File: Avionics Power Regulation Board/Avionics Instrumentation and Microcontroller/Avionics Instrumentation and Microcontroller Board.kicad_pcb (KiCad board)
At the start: 2 copper layers, 101.9 x 63.6 mm, 18 parts, among them J1 Conn_01x04_Socket, J2 Conn_01x07_Socket, J3 Conn_01x06_Socket, J4 Conn_01x08_Socket, J5 Conn_01x05_Socket, J6 Conn_02x07_Odd_Even, J7 Micro_SD_Card_Det1, U1 SC0917

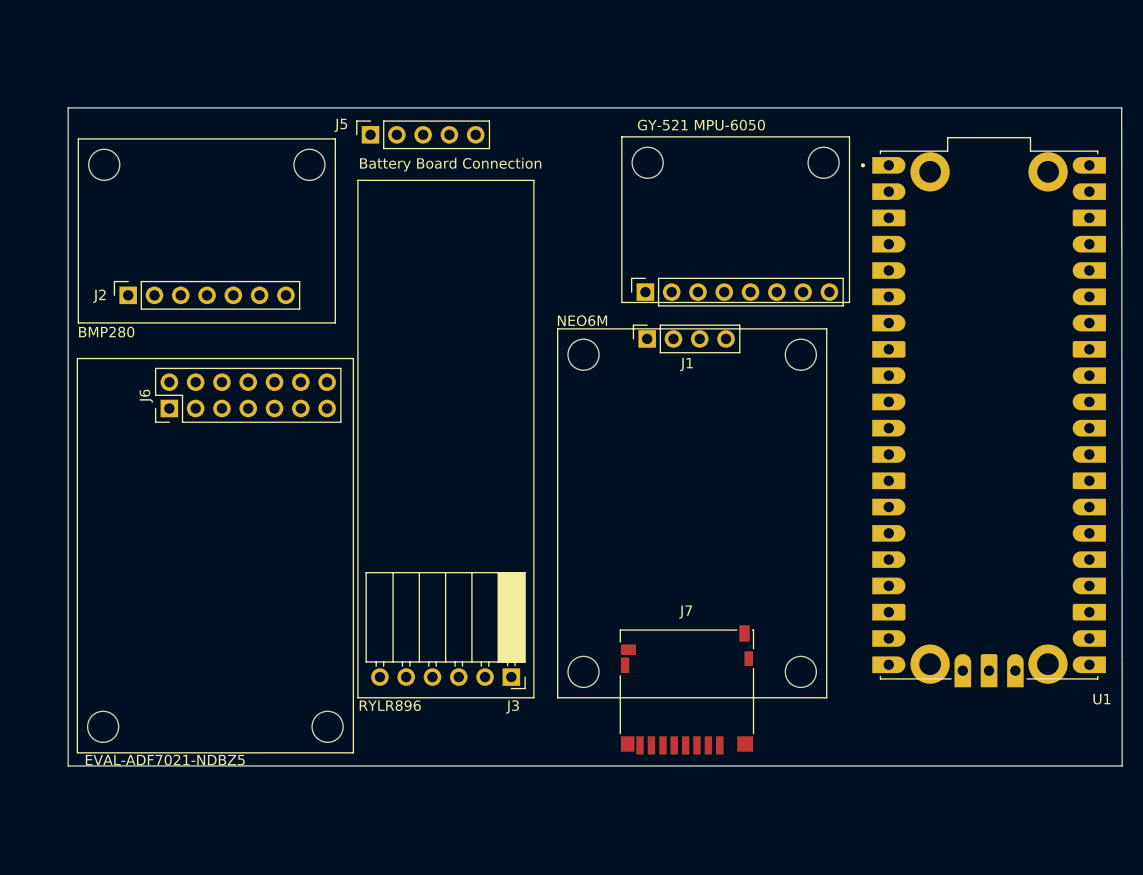
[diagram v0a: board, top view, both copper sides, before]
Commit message: Small Changes
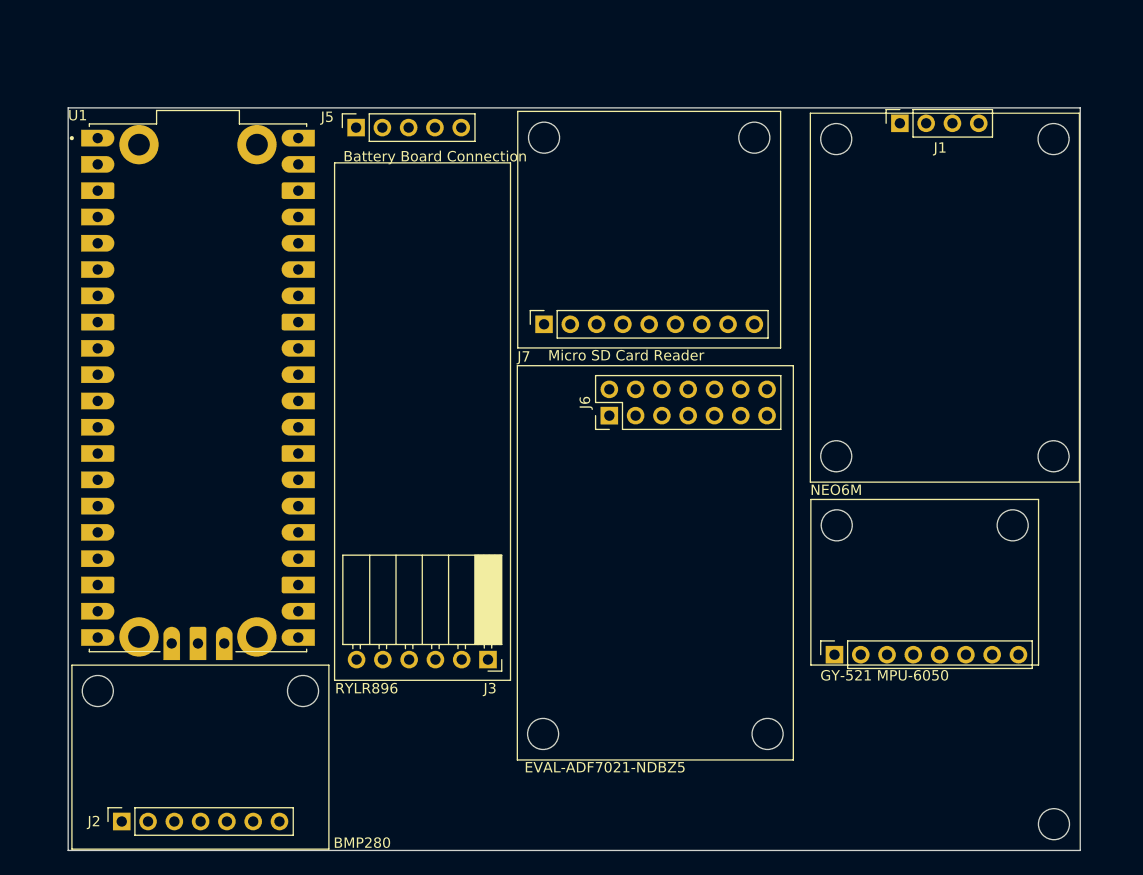
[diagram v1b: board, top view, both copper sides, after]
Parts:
- added H12: MountingHole, MountingHole:MountingHole_2.1mm, F.Cu at (80.3, 29.0)
- added H13: MountingHole, MountingHole:MountingHole_2.1mm, F.Cu at (100.6, 29.0)
- added H2: MountingHole, MountingHole:MountingHole_2.1mm, F.Cu at (129.5, 95.4)
- J7: value Micro_SD_Card_Det1 -> Conn_01x09_Socket; footprint Connector_Card:microSD_HC_Hirose_DM3D-SF -> Connector_PinSocket_2.54mm:PinSocket_1x09_P2.54mm_Vertical
- moved U1 76.5 mm to (46.8, 53.2)
- moved H1 50.8 mm to (37.1, 82.5)
- moved H7 50.8 mm to (57.0, 82.5)
- moved J2 50.8 mm to (39.5, 95.1)
- moved H11 42.5 mm to (80.2, 86.7)
- moved J6 42.5 mm to (86.6, 55.9)
- moved H8 42.5 mm to (101.9, 86.7)
- moved H10 39.5 mm to (125.5, 66.5)
- moved H9 39.5 mm to (108.5, 66.5)
- moved J4 39.5 mm to (108.3, 79.0)
- moved J7 37.9 mm to (80.3, 47.1), turned to 90 degrees
- moved H3 32.1 mm to (108.5, 29.2)
- moved H5 32.1 mm to (129.5, 29.2)
- moved H4 32.1 mm to (108.5, 59.8)
- moved H6 32.1 mm to (129.5, 59.8)
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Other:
- board size 101.9 x 63.6 mm -> 97.8 x 71.8 mm

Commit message: more changes
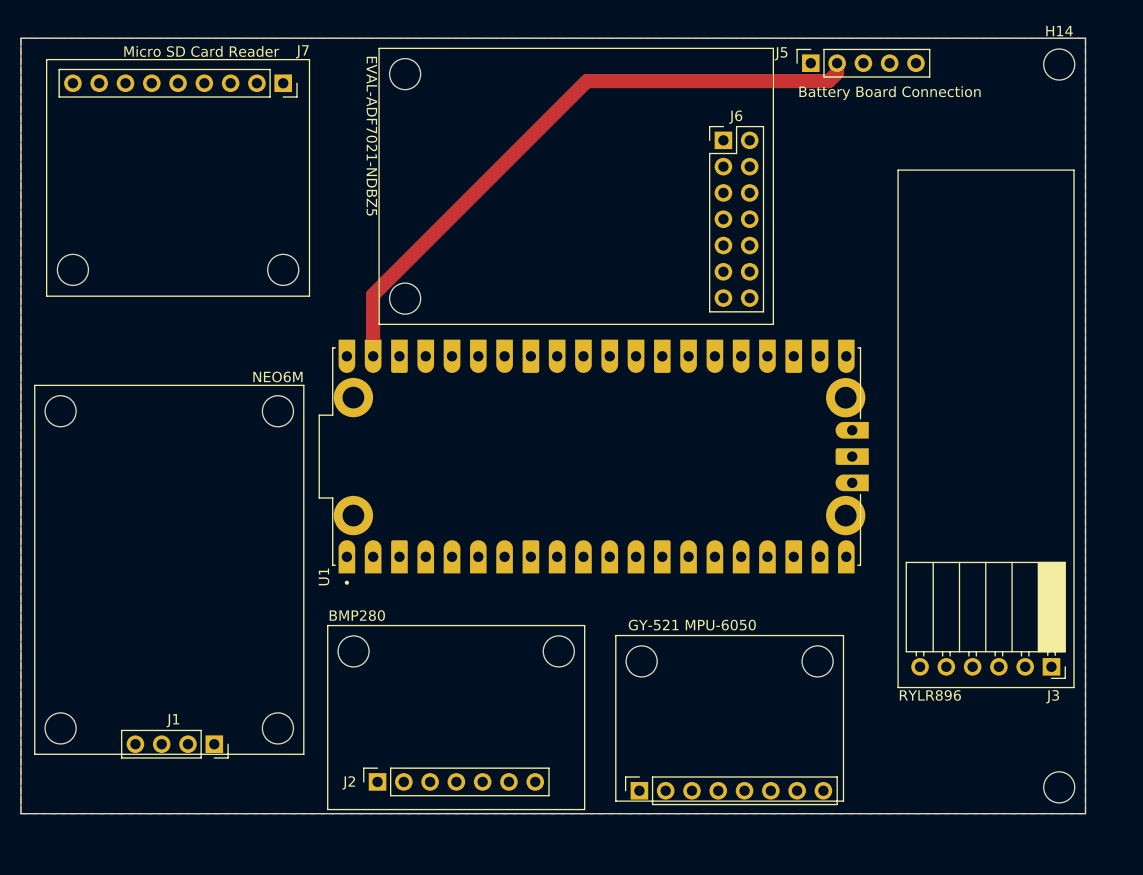
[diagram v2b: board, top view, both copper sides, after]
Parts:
- added G***: LOGO, AIAA Logo:AIAA_Fresno_Logo_20mm_positive, B.Cu at (85.6, 34.2)
- added H14: MountingHole, MountingHole:MountingHole_2.1mm, F.Cu at (130.0, 22.0)
- added REF**: KiCad-Logo2_12mm_SilkScreen, Symbol:KiCad-Logo2_12mm_SilkScreen, B.Cu at (85.6, 58.4)
- moved H5 111.6 mm to (33.5, 86.1), turned to 180 degrees
- moved H6 96.0 mm to (33.5, 55.5), turned to 180 degrees
- moved J1 89.4 mm to (48.4, 87.7), turned to -90 degrees
- moved H3 78.4 mm to (54.5, 86.1), turned to 180 degrees
- moved H13 67.1 mm to (34.7, 41.8), turned to 180 degrees
- moved H11 65.1 mm to (66.8, 22.9), turned to -90 degrees
- moved H8 54.7 mm to (66.8, 44.6), turned to -90 degrees
- moved J3 54.5 mm to (129.3, 80.2)
- moved H4 54.1 mm to (54.5, 55.5), turned to 180 degrees
- moved J5 44.4 mm to (106.0, 21.8)
- moved U1 39.1 mm to (85.3, 59.9), turned to 90 degrees
- moved J7 34.3 mm to (55.1, 23.8), turned to -90 degrees
- moved J6 28.8 mm to (97.6, 29.3), turned to 0 degrees
- moved H12 28.3 mm to (55.1, 41.8), turned to 180 degrees
- moved H1 25.0 mm to (61.9, 78.7)
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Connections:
- J1 pad 1: unconnected-(J1-Pin_1-Pad1) -> /3.3V
- J1 pad 4: unconnected-(J1-Pin_4-Pad4) -> GNDREF
- J2 pad 1: unconnected-(J2-Pin_1-Pad1) -> /3.3V
- J2 pad 3: unconnected-(J2-Pin_3-Pad3) -> GNDREF
- J3 pad 1: unconnected-(J3-Pin_1-Pad1) -> /3.3V
- J3 pad 6: unconnected-(J3-Pin_6-Pad6) -> GNDREF
- J4 pad 1: unconnected-(J4-Pin_1-Pad1) -> /3.3V
- J4 pad 2: unconnected-(J4-Pin_2-Pad2) -> GNDREF
- J5 pad 1: unconnected-(J5-Pin_1-Pad1) -> GNDREF
- J5 pad 2: unconnected-(J5-Pin_2-Pad2) -> /Vin
- J7 pad 1: unconnected-(J7-Pin_1-Pad1) -> /3.3V
- J7 pad 2: unconnected-(J7-Pin_2-Pad2) -> GNDREF
- U1 pad 36: unconnected-(U1-3V3_OUT-Pad36) -> /3.3V
- U1 pad 39: unconnected-(U1-VSYS-Pad39) -> /Vin
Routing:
- net /Vin: track 0.00 -> 60.6 mm
- added copper zone on F.Cu, net /3.3V
- added copper zone on B.Cu, net GNDREF
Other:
- board size 97.8 x 71.8 mm -> 102.9 x 74.9 mm
- board text added: "Fresno State AIAA Nasa SLI Avionics Board Designed by the Fresno State AIAA Avionics Team Version 1.0"
